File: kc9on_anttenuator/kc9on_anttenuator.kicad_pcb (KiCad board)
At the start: 2 copper layers, 30 x 60 mm, 20 parts, among them J1 9v Battery, J2 Antenna, J3 Radio, Q1 MMBF5457, SW1 SW_SPDT, Y1 4.000MHz

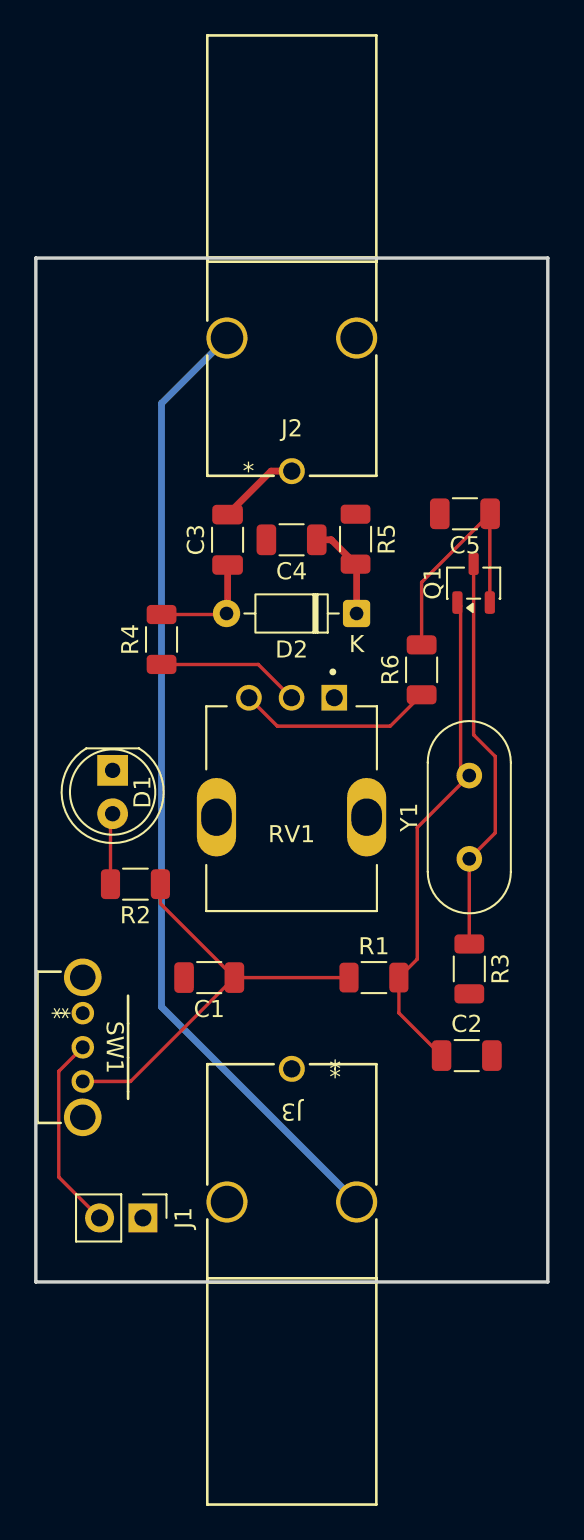
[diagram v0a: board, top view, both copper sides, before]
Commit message: Through hole madness
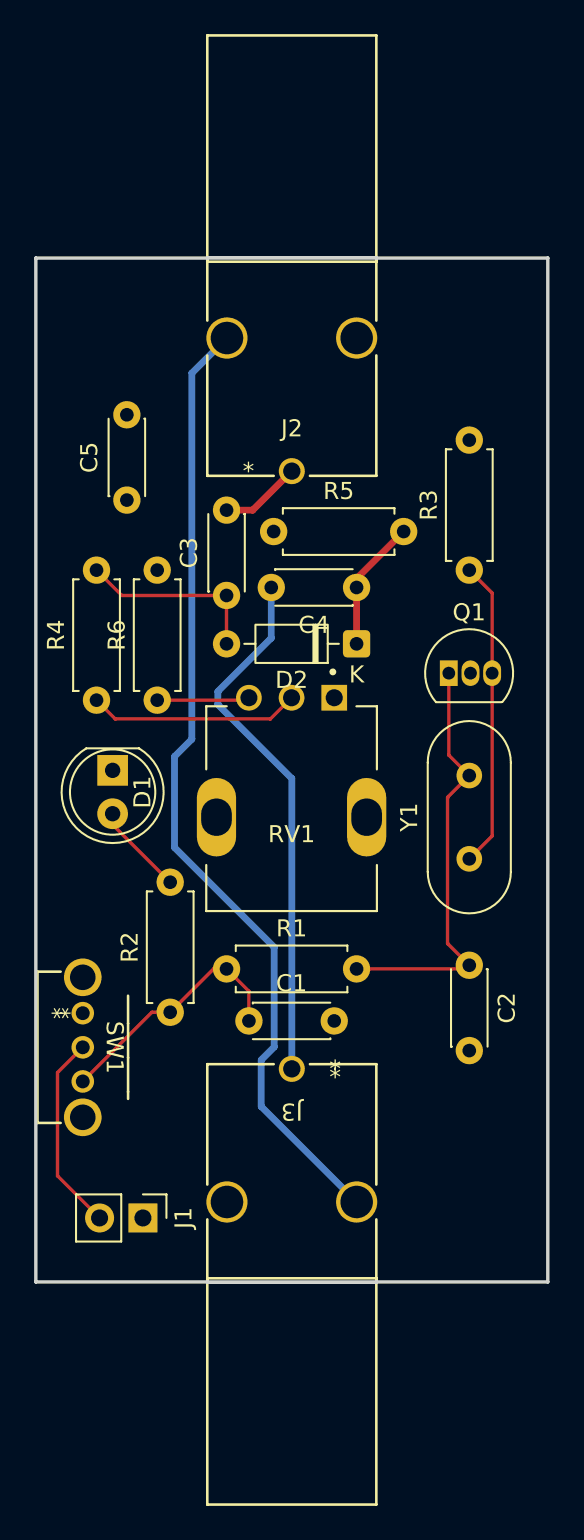
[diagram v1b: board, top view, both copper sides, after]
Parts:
- C1, C3, C4, C5: footprint Capacitor_SMD:C_1206_3216Metric -> Capacitor_THT:C_Disc_D4.3mm_W1.9mm_P5.00mm
- C2: value 15pf -> 15pF; footprint Capacitor_SMD:C_1206_3216Metric -> Capacitor_THT:C_Disc_D4.3mm_W1.9mm_P5.00mm
- Q1: value MMBF5457 -> J113; footprint Package_TO_SOT_SMD:SOT-23-3 -> Package_TO_SOT_THT:TO-92L_Inline
- R1, R2, R3, R4, R5: footprint Resistor_SMD:R_1206_3216Metric -> Resistor_THT:R_Axial_DIN0207_L6.3mm_D2.5mm_P7.62mm_Horizontal
- R6: value 2.2K -> 2.2k; footprint Resistor_SMD:R_1206_3216Metric -> Resistor_THT:R_Axial_DIN0207_L6.3mm_D2.5mm_P7.62mm_Horizontal
- moved R3 23.4 mm to (167.4, 88.8), turned to 90 degrees
- moved C5 19.8 mm to (147.3, 84.7), turned to 90 degrees
- moved R6 15.6 mm to (149.1, 96.4)
- moved R1 8.65 mm to (153.2, 112.2)
- moved R2 7.78 mm to (149.9, 114.7), turned to 90 degrees
- moved Q1 5.47 mm to (166.2, 94.8), turned to 0 degrees
- moved C2 5.30 mm to (167.4, 111.9), turned to -90 degrees
- moved R4 5.21 mm to (145.6, 96.4)
- moved R5 4.82 mm to (155.9, 86.5), turned to 0 degrees
- moved C4 4.72 mm to (160.8, 89.8)
- moved C1 3.44 mm to (154.5, 115.2), turned to 0 degrees
- moved C3 3.26 mm to (153.2, 90.3)
- moved D2 1.78 mm to (160.8, 93.1)
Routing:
- net Net-(J3-In): track 0.00 -> 31.3 mm
- net Net-(Q1-S): track 14.6 -> 0.00 mm
- net Net-(SW1-C): track 25.4 -> 14.7 mm
- net Net-(R6-Pad1): track 11.6 -> 5.43 mm
- net Net-(Q1-G): track 23.4 -> 18.0 mm
- net Net-(D2-A): track 6.70 -> 11.1 mm
- net Net-(Q1-D): track 29.6 -> 25.4 mm
- net Net-(R4-Pad1): track 8.43 -> 12.4 mm
- net Net-(D2-K): track 5.78 -> 7.72 mm
- net Net-(D1-A): track 4.18 -> 5.41 mm
